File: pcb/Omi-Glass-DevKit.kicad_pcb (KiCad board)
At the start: 2 copper layers, 24.4 x 16.5 mm, 12 parts, among them J1 Conn_01x02, J2 Conn_01x02, SW1 SW_Push, U1 NCP163AFCS280T2G, U2 NCP163AFCT180T2G

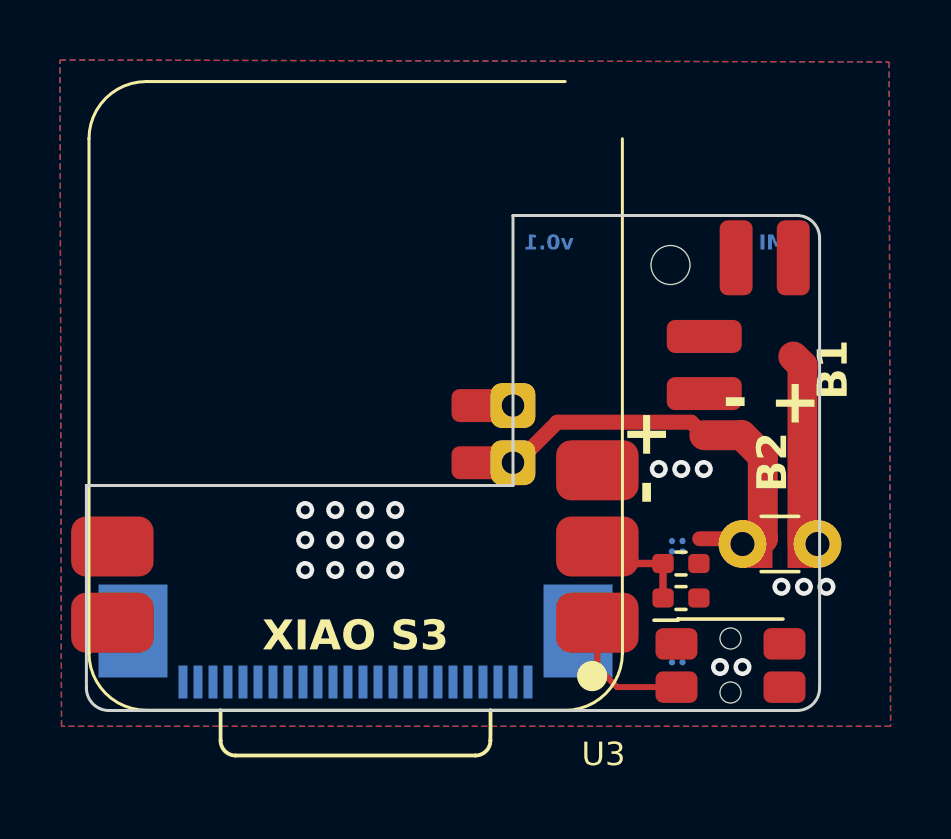
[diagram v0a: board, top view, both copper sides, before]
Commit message: push R0.0 design for V3 glasses
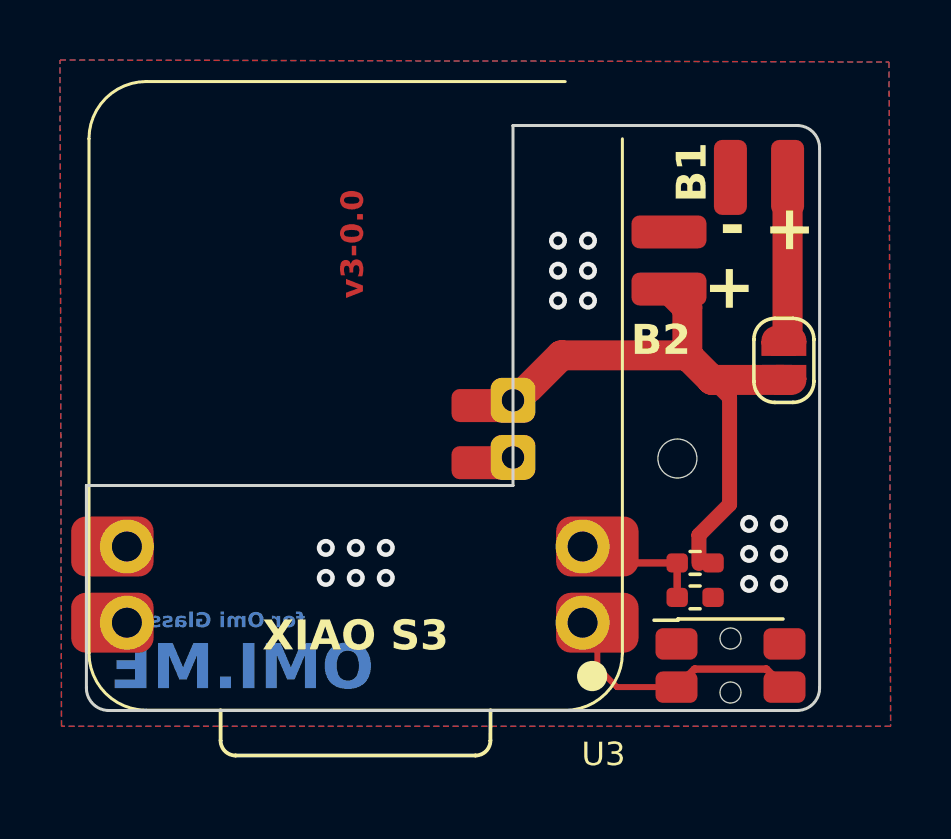
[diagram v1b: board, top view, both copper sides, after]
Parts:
- removed the REF** at (0.00, 8.20)
- removed TH1: Thermistor_NTC, Capacitor_THT:C_Disc_D3.0mm_W1.6mm_P2.50mm
- removed U1: NCP163AFCS280T2G, Package_CSP:WLCSP-4_0.64x0.64mm_P0.35mm
- removed U2: NCP163AFCT180T2G, Package_CSP:WLCSP-4_0.64x0.64mm_P0.35mm
- added JP1: Jumper_2_Open, Jumper:SolderJumper-2_P1.3mm_Open_RoundedPad1.0x1.5mm, F.Cu at (14.3, -1.17)
- moved REF** 6.45 mm to (10.7, 2.10)
- moved J2 3.68 mm to (10.4, -4.50), turned to -90 degrees
- moved J1 2.69 mm to (13.4, -7.27)
- moved R1 0.47 mm to (11.3, 5.58)
- moved R2 0.47 mm to (11.3, 6.73)
- turned J3 to 90 degrees
- renumbered J2 to J3
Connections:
- U3 pad 3: unconnected-(U3-D2-Pad3) -> (no net)
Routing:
- net LOAD: track 13.4 -> 18.6 mm
- net POWER: track 4.40 -> 8.50 mm
- net VBAT1: track 6.38 -> 5.50 mm
- net GND: vias 20 -> 18
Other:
- board size 24.4 x 16.5 mm -> 24.4 x 19.5 mm
- board text added: "for Omi Glass v3"
- board text added: "v3-0.0"
- board text removed: "Design by Alex Lynd"
- board text removed: "OMI"
- board text removed: "v0.1"
